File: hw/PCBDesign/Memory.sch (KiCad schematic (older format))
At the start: 18 parts, among them U4 AT25SF081, U5 AT24C256

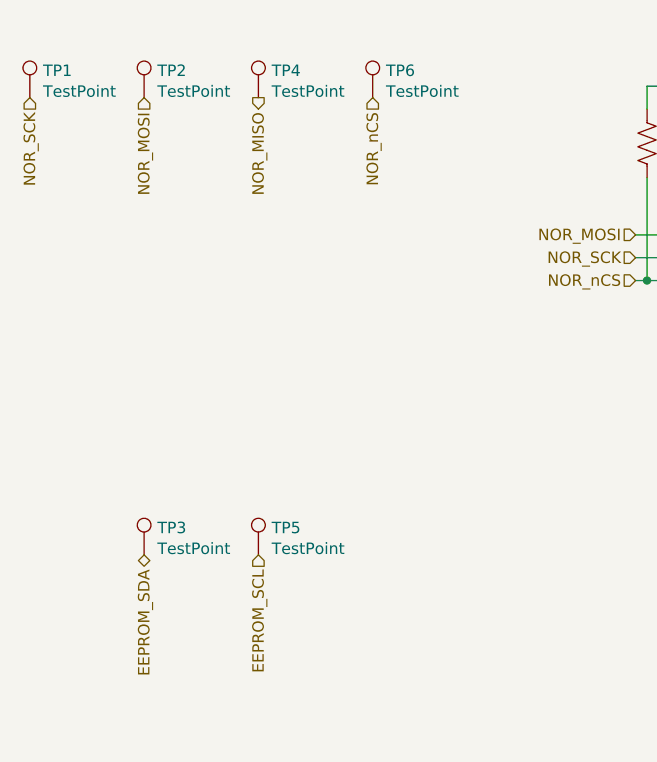
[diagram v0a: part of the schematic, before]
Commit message: Add more work on PCB v2 design
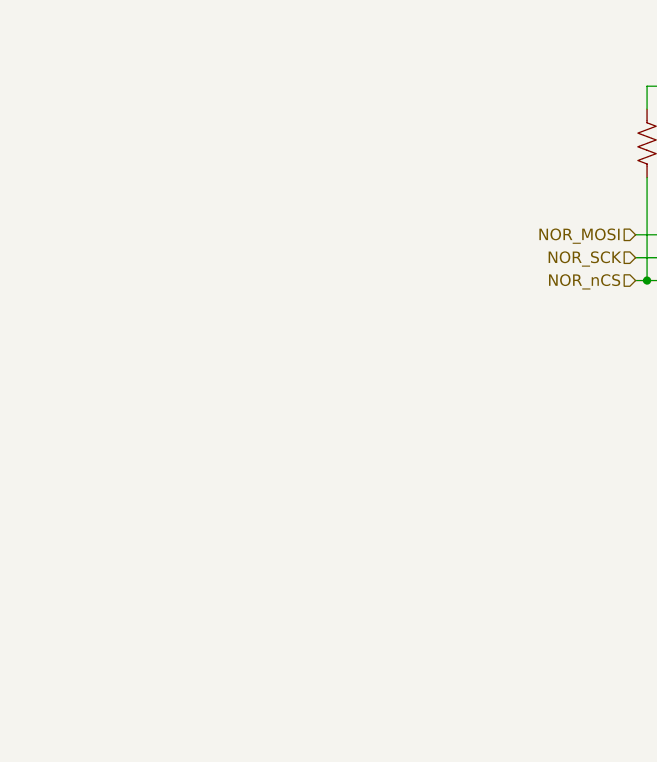
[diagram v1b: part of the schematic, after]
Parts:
- removed TP1, TP2, TP3, TP4, TP5, TP6: TestPoint, TestPoint:TestPoint_Pad_2.5x2.5mm, symbol Connector:TestPoint
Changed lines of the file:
@@
 Wire Wire Line
 	4900 4300 5550 4300
-$Comp
-L Connector:TestPoint TP2
-U 1 1 605C449A
-P 2500 2000
-F 0 "TP2" H 2558 2118 50  0000 L CNN
-F 1 "TestPoint" H 2558 2027 50  0000 L CNN
-F 2 "TestPoint:TestPoint_Pad_2.5x2.5mm" H 2700 2000 50  0001 C CNN
-F 3 "~" H 2700 2000 50  0001 C CNN
-	1    2500 2000
-	1    0    0    -1
-$EndComp
-$Comp
-L Connector:TestPoint TP4
-U 1 1 605C46E9
-P 3000 2000
-F 0 "TP4" H 3058 2118 50  0000 L CNN
-F 1 "TestPoint" H 3058 2027 50  0000 L CNN
-F 2 "TestPoint:TestPoint_Pad_2.5x2.5mm" H 3200 2000 50  0001 C CNN
-F 3 "~" H 3200 2000 50  0001 C CNN
-	1    3000 2000
-	1    0    0    -1
-$EndComp
-$Comp
-L Connector:TestPoint TP6
-U 1 1 605C4942
-P 3500 2000
-F 0 "TP6" H 3558 2118 50  0000 L CNN
-F 1 "TestPoint" H 3558 2027 50  0000 L CNN
-F 2 "TestPoint:TestPoint_Pad_2.5x2.5mm" H 3700 2000 50  0001 C CNN
-F 3 "~" H 3700 2000 50  0001 C CNN
-	1    3500 2000
-	1    0    0    -1
-$EndComp
-$Comp
-L Connector:TestPoint TP1
-U 1 1 605C4AD4
-P 2000 2000
-F 0 "TP1" H 2058 2118 50  0000 L CNN
-F 1 "TestPoint" H 2058 2027 50  0000 L CNN
-F 2 "TestPoint:TestPoint_Pad_2.5x2.5mm" H 2200 2000 50  0001 C CNN
-F 3 "~" H 2200 2000 50  0001 C CNN
-	1    2000 2000
-	1    0    0    -1
-$EndComp
-$Comp
-L Connector:TestPoint TP3
-U 1 1 605C4DEB
-P 2500 4000
-F 0 "TP3" H 2558 4118 50  0000 L CNN
-F 1 "TestPoint" H 2558 4027 50  0000 L CNN
-F 2 "TestPoint:TestPoint_Pad_2.5x2.5mm" H 2700 4000 50  0001 C CNN
-F 3 "~" H 2700 4000 50  0001 C CNN
-	1    2500 4000
-	1    0    0    -1
-$EndComp
-$Comp
-L Connector:TestPoint TP5
-U 1 1 605C5090
-P 3000 4000
-F 0 "TP5" H 3058 4118 50  0000 L CNN
-F 1 "TestPoint" H 3058 4027 50  0000 L CNN
-F 2 "TestPoint:TestPoint_Pad_2.5x2.5mm" H 3200 4000 50  0001 C CNN
-F 3 "~" H 3200 4000 50  0001 C CNN
-	1    3000 4000
-	1    0    0    -1
-$EndComp
-Text HLabel 3500 2000 3    50   Input ~ 0
-NOR_nCS
-Text HLabel 3000 2000 3    50   Output ~ 0
-NOR_MISO
-Text HLabel 2500 2000 3    50   Input ~ 0
-NOR_MOSI
-Text HLabel 2500 4000 3    50   BiDi ~ 0
-EEPROM_SDA
-Text HLabel 3000 4000 3    50   Input ~ 0
-EEPROM_SCL
-Text HLabel 2000 2000 3    50   Input ~ 0
-NOR_SCK
 $EndSCHEMATC
